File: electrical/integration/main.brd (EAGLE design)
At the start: 168 x 104 mm, 115 parts

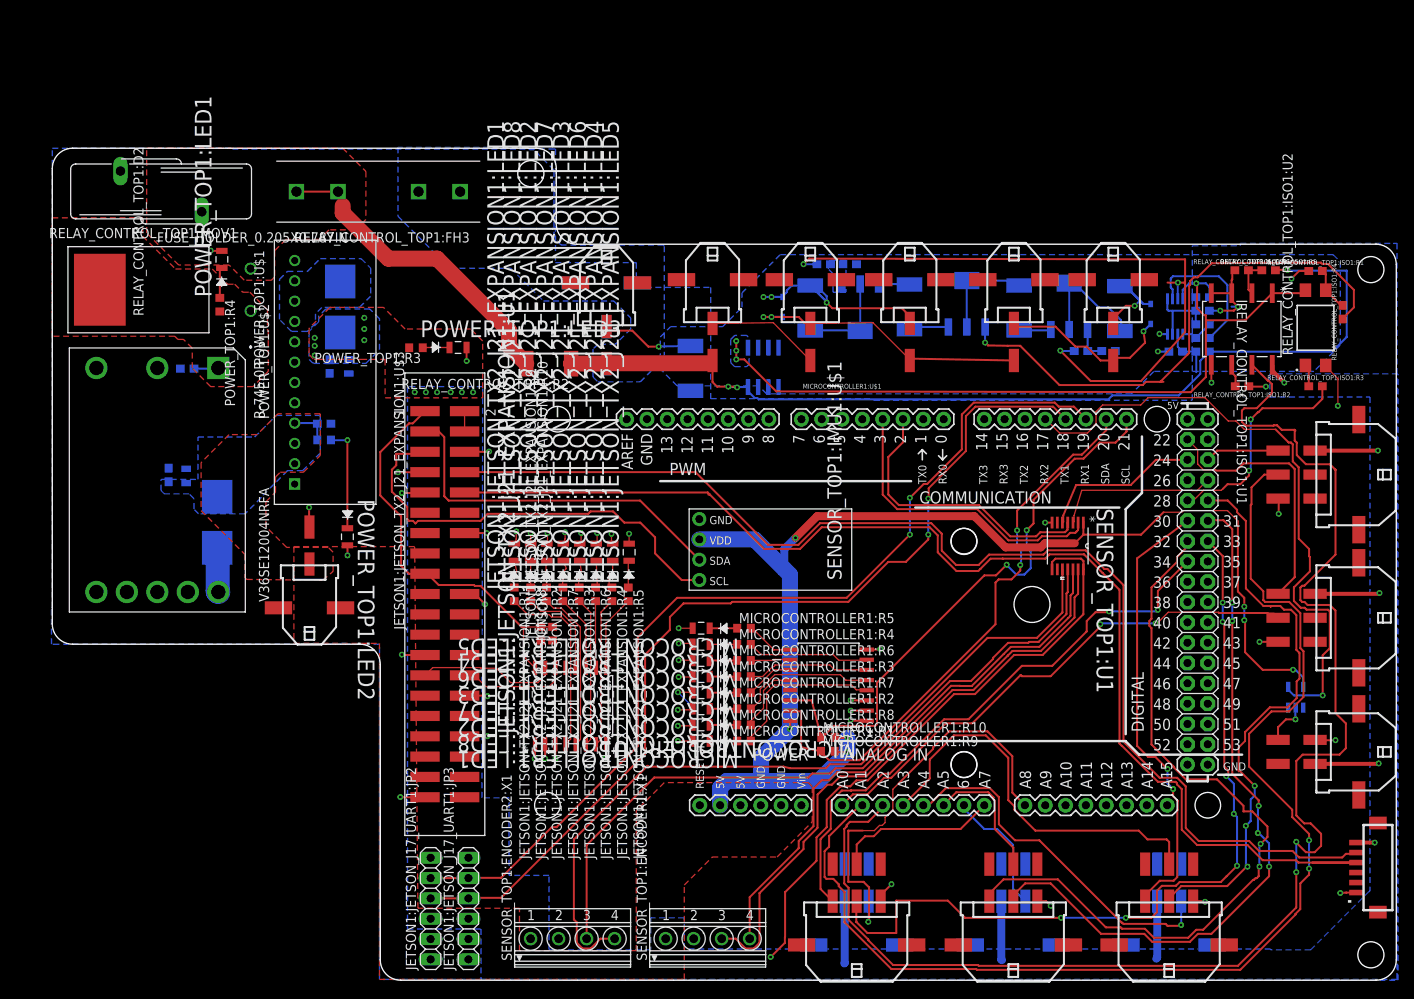
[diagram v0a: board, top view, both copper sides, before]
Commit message: increment
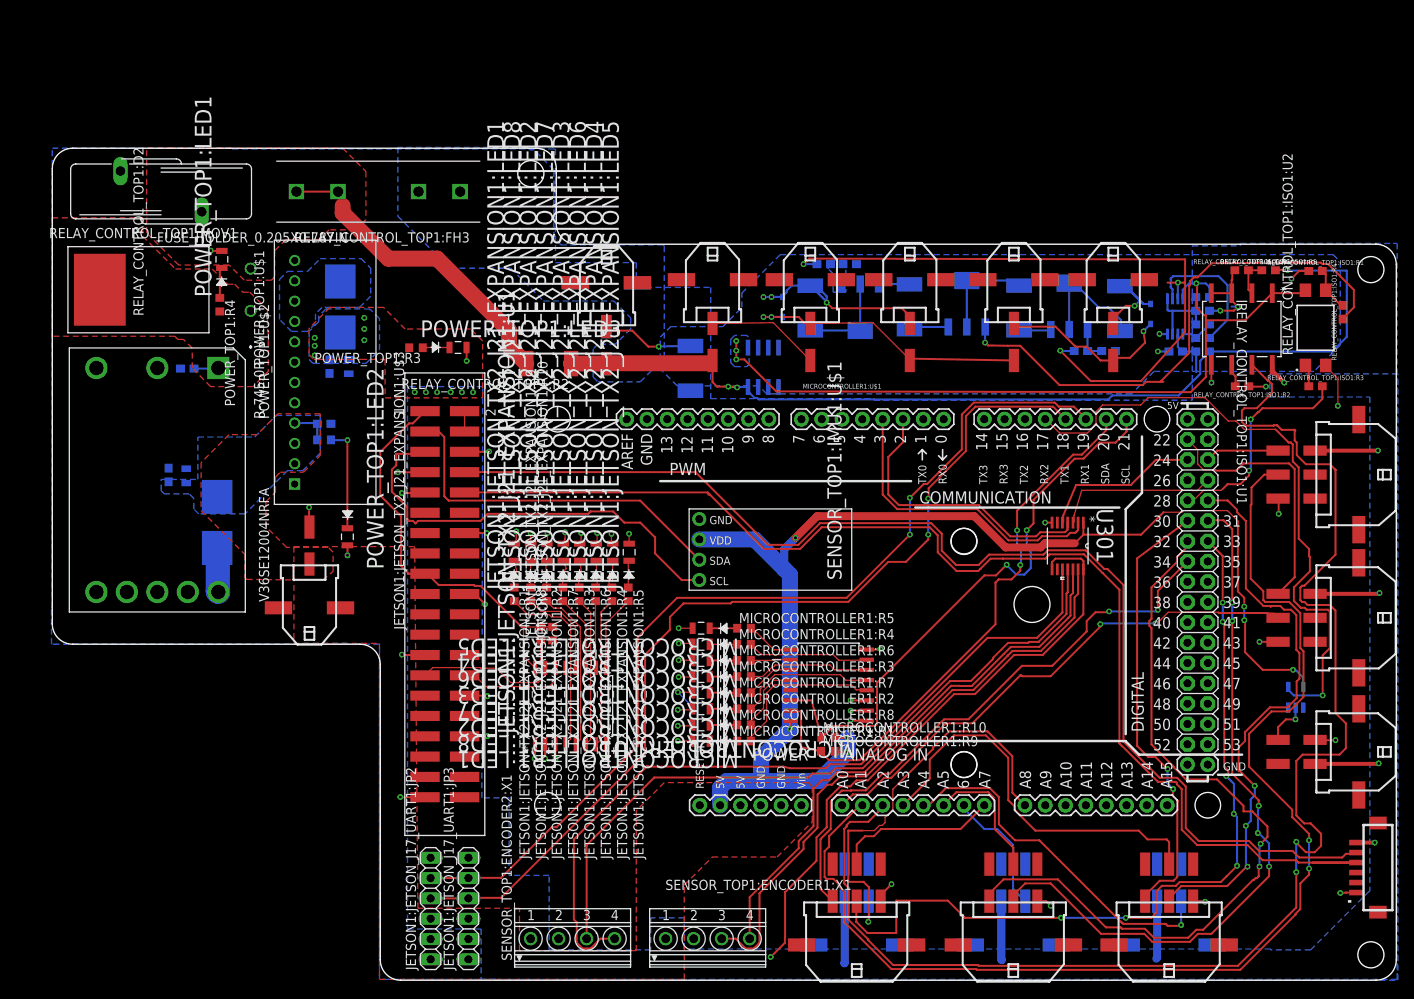
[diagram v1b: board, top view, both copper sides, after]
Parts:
- renumbered JETSON1:X1 to X101, SENSOR_TOP1:U1 to U301
